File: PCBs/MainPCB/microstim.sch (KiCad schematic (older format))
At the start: 105 parts, among them J1 Conn_02x08_Counter_Clockwise, J2 Conn_Coaxial, J3 Conn_Coaxial, J4 Screw_Terminal_01x02, J5 Screw_Terminal_01x02, J6 Screw_Terminal_01x02, J7 Conn_Coaxial, J8 Screw_Terminal_01x02, J9 Conn_Coaxial, SW1 SW_Push, U1 Teensy3.5, U10 AD8276, U11 INA826, U12 DG509ACWE, U13 CC3-0512DF-E, U14 ISO7760, U15 ISO7341C, U16 L78L05_SO8, U17 AD5752, U18 AD7321, U19 AD1582, U2 CC3-0512DF-E, U20 OPA197, U21 AD8276, U22 INA826, U23 DG509ACWE, U3 ISO7760, U4 ISO7341C, U5 L78L05_SO8, U6 AD5752, U7 AD7321, U8 AD1582, U9 OPA197

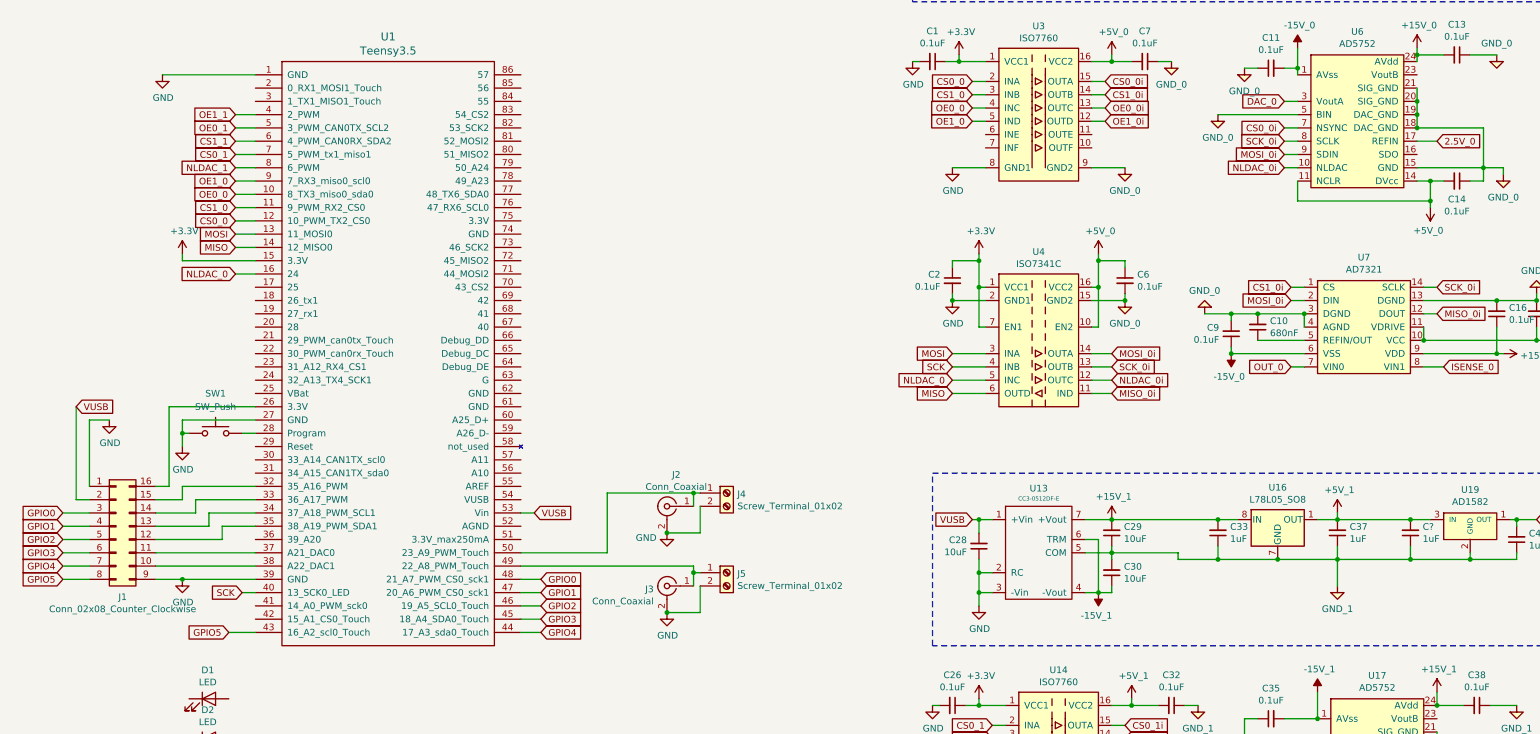
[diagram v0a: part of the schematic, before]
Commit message: getting darn close to done with layout.
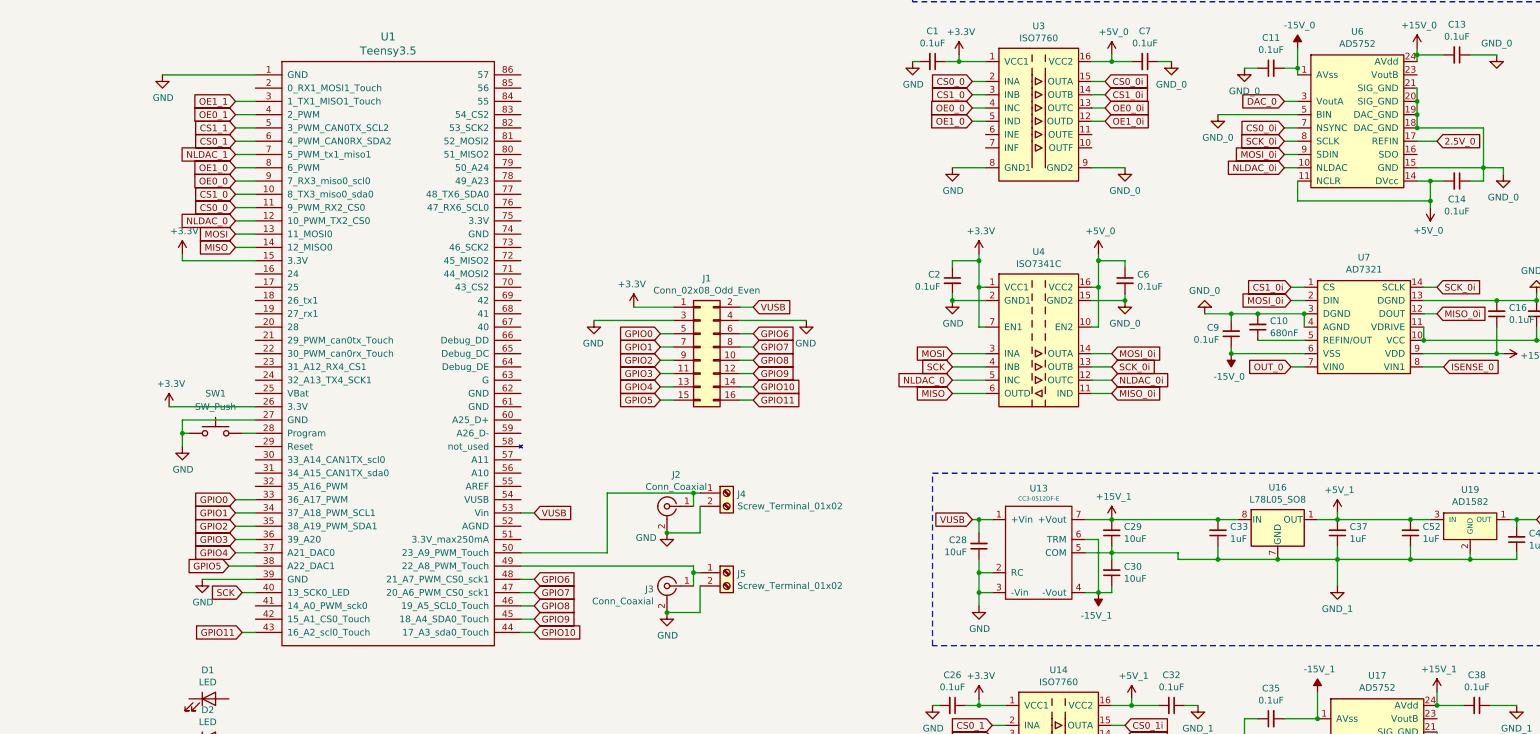
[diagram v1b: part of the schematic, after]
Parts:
- removed J1: Conn_02x08_Counter_Clockwise, Connector_Multicomp:Multicomp_MC9A22-1634_2x08_P2.54mm_Horizontal, symbol Connector_Generic:Conn_02x08_Counter_Clockwise
- added J1: Conn_02x08_Odd_Even, Connector_Multicomp:Multicomp_MC9A22-1634_2x08_P2.54mm_Horizontal, symbol Connector_Generic:Conn_02x08_Odd_Even
- gave numbers to parts that had none: 1
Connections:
- net +3V3: now also U1.26 (3.3V), J1.1 (Pin_1)
- net CS0_0: now also U1.11 (9_PWM_RX2_CS0); no longer U1.12 (10_PWM_TX2_CS0)
- net CS0_1: now also U1.6 (4_PWM_CAN0RX_SDA2); no longer U1.7 (5_PWM_tx1_miso1)
- net CS1_0: now also U1.10 (8_TX3_miso0_sda0); no longer U1.11 (9_PWM_RX2_CS0)
- net CS1_1: now also U1.5 (3_PWM_CAN0TX_SCL2); no longer U1.6 (4_PWM_CAN0RX_SDA2)
- net GND: now also J1.3 (Pin_3), J1.4 (Pin_4)
- net GPIO0: now also U1.33 (36_A17_PWM), J1.5 (Pin_5); no longer U1.48 (21_A7_PWM_CS0_sck1)
- net GPIO1: now also U1.34 (37_A18_PWM_SCL1), J1.7 (Pin_7); no longer U1.47 (20_A6_PWM_CS0_sck1)
- net GPIO2: now also U1.35 (38_A19_PWM_SDA1), J1.9 (Pin_9); no longer U1.46 (19_A5_SCL0_Touch)
- net GPIO3: now also U1.36 (39_A20), J1.11 (Pin_11); no longer U1.45 (18_A4_SDA0_Touch)
- net GPIO4: now also U1.37 (A21_DAC0), J1.13 (Pin_13); no longer U1.44 (17_A3_sda0_Touch)
- net GPIO5: now also U1.38 (A22_DAC1), J1.15 (Pin_15); no longer U1.43 (16_A2_scl0_Touch)
- net NLDAC_0: now also U1.12 (10_PWM_TX2_CS0); no longer U1.16 (24)
- net NLDAC_1: now also U1.7 (5_PWM_tx1_miso1); no longer U1.8 (6_PWM)
- net OE0_0: now also U1.9 (7_RX3_miso0_scl0); no longer U1.10 (8_TX3_miso0_sda0)
- net OE0_1: now also U1.4 (2_PWM); no longer U1.5 (3_PWM_CAN0TX_SCL2)
- net OE1_0: now also U1.8 (6_PWM); no longer U1.9 (7_RX3_miso0_scl0)
- net OE1_1: now also U1.3 (1_TX1_MISO1_Touch); no longer U1.4 (2_PWM)
- net VUSB: now also J1.2 (Pin_2)
- new net GPIO10: J1.14 (Pin_14), U1.44 (17_A3_sda0_Touch)
- new net GPIO11: J1.16 (Pin_16), U1.43 (16_A2_scl0_Touch)
- new net GPIO6: J1.6 (Pin_6), U1.48 (21_A7_PWM_CS0_sck1)
- new net GPIO7: J1.8 (Pin_8), U1.47 (20_A6_PWM_CS0_sck1)
- new net GPIO8: J1.10 (Pin_10), U1.46 (19_A5_SCL0_Touch)
- new net GPIO9: J1.12 (Pin_12), U1.45 (18_A4_SDA0_Touch)
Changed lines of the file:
@@
 Text GLabel 7350 1900 0    50   Input ~ 0
 OE0_0
-Text GLabel 1800 3150 0    50   Input ~ 0
+Text GLabel 1800 2750 0    50   Input ~ 0
 NLDAC_0
 $Comp
@@
 Wire Wire Line
 	8250 2350 8500 2350
-Text GLabel 1800 2650 0    50   Input ~ 0
+Text GLabel 1800 2550 0    50   Input ~ 0
 CS1_0
-Text GLabel 1800 2750 0    50   Input ~ 0
+Text GLabel 1800 2650 0    50   Input ~ 0
 CS0_0
 Wire Wire Line
@@
 Wire Wire Line
 	16750 4850 16900 4850
-Text GLabel 1800 2450 0    50   Input ~ 0
+Text GLabel 1800 2350 0    50   Input ~ 0
 OE1_0
-Text GLabel 1800 2550 0    50   Input ~ 0
+Text GLabel 1800 2450 0    50   Input ~ 0
 OE0_0
 Wire Wire Line
@@
 Wire Wire Line
 	1850 4350 1950 4350
-$Comp
-L Connector_Generic:Conn_02x08_Counter_Clockwise J1
-U 1 1 5CBED068
-P 900 5050
-F 0 "J1" H 950 4517 50  0000 C CNN
-F 1 "Conn_02x08_Counter_Clockwise" H 950 4426 50  0000 C CNN
-F 2 "Connector_Multicomp:Multicomp_MC9A22-1634_2x08_P2.54mm_Horizontal" H 900 5050 50  0001 C CNN
-F 3 "~" H 900 5050 50  0001 C CNN
-	1    900  5050
-	1    0    0    -1
-$EndComp
-Wire Wire Line
-	700  4250 700  4750
-Wire Wire Line
-	700  4850 600  4850
-Wire Wire Line
-	600  4850 600  4150
 Wire Wire Line
-	500  4950 700  4950
+	5000 3600 5100 3600
 Wire Wire Line
-	500  5050 700  5050
+	5000 3700 5100 3700
 Wire Wire Line
-	500  5150 700  5150
+	5000 3800 5100 3800
 Wire Wire Line
-	500  5250 700  5250
+	5000 3900 5100 3900
 Wire Wire Line
-	500  5350 700  5350
+	5000 4000 5100 4000
 Wire Wire Line
-	700  5450 500  5450
-Wire Wire Line
-	1950 5350 1200 5350
-Wire Wire Line
-	1200 5250 1950 5250
+	5100 4100 5000 4100
 Wire Wire Line
 	9950 150  10500 150
@@
 	1    0    0    -1
 $EndComp
-$Comp
-L power:GND #PWR01
-U 1 1 5C5D1E51
-P 850 4250
-F 0 "#PWR01" H 850 4000 50  0001 C CNN
-F 1 "GND" H 855 4077 50  0000 C CNN
-F 2 "" H 850 4250 50  0001 C CNN
-F 3 "" H 850 4250 50  0001 C CNN
-	1    850  4250
-	1    0    0    -1
-$EndComp
-Wire Wire Line
-	700  4250 850  4250
 Wire Wire Line
 	1950 4250 1400 4250
@@
 	1400 4350 1400 4450
 Wire Wire Line
-	1950 5050 1700 5050
-Wire Wire Line
-	1700 5050 1700 5150
-Wire Wire Line
-	1700 5150 1200 5150
-Wire Wire Line
-	1200 5050 1600 5050
-Wire Wire Line
-	1600 5050 1600 4950
-Wire Wire Line
-	1600 4950 1950 4950
-Wire Wire Line
-	1200 4950 1500 4950
-Wire Wire Line
-	1500 4950 1500 4850
-Wire Wire Line
-	1500 4850 1950 4850
-Wire Wire Line
-	1200 4850 1400 4850
-Wire Wire Line
-	1400 4850 1400 4750
-Wire Wire Line
-	1950 4750 1400 4750
-Wire Wire Line
-	1200 4750 1300 4750
-Wire Wire Line
-	1300 4750 1300 4150
-Wire Wire Line
 	1300 4150 1950 4150
-Text GLabel 600  4150 2    50   Input ~ 0
+Text GLabel 5700 3400 2    50   Input ~ 0
 VUSB
-Wire Wire Line
-	1200 5450 1400 5450
 $Comp
 L power:GND #PWR05
 U 1 1 5C9B26A7
-P 1400 5450
-F 0 "#PWR05" H 1400 5200 50  0001 C CNN
-F 1 "GND" H 1405 5277 50  0000 C CNN
-F 2 "" H 1400 5450 50  0001 C CNN
-F 3 "" H 1400 5450 50  0001 C CNN
-	1    1400 5450
-	1    0    0    -1
+P 4500 3500
+F 0 "#PWR05" H 4500 3250 50  0001 C CNN
+F 1 "GND" H 4505 3327 50  0000 C CNN
+F 2 "" H 4500 3500 50  0001 C CNN
+F 3 "" H 4500 3500 50  0001 C CNN
+	1    4500 3500
+	-1   0    0    -1
 $EndComp
-Connection ~ 1400 5450
-Wire Wire Line
-	1400 5450 1950 5450
-Text GLabel 500  5450 0    50   Input ~ 0
+Text GLabel 5000 4100 0    50   Input ~ 0
 GPIO5
-Text GLabel 500  5350 0    50   Input ~ 0
+Text GLabel 5000 4000 0    50   Input ~ 0
 GPIO4
-Text GLabel 500  5250 0    50   Input ~ 0
+Text GLabel 5000 3900 0    50   Input ~ 0
 GPIO3
-Text GLabel 500  5050 0    50   Input ~ 0
+Text GLabel 5000 3700 0    50   Input ~ 0
 GPIO1
-Text GLabel 500  5150 0    50   Input ~ 0
+Text GLabel 5000 3800 0    50   Input ~ 0
 GPIO2
-Text GLabel 500  4950 0    50   Input ~ 0
+Text GLabel 5000 3600 0    50   Input ~ 0
 GPIO0
-Text GLabel 1750 5850 0    50   Input ~ 0
+Text GLabel 1750 5350 0    50   Input ~ 0
 GPIO5
-Text GLabel 4100 5850 2    50   Input ~ 0
+Text GLabel 1800 5250 0    50   Input ~ 0
 GPIO4
-Text GLabel 4100 5750 2    50   Input ~ 0
+Text GLabel 1800 5150 0    50   Input ~ 0
 GPIO3
-Text GLabel 4100 5550 2    50   Input ~ 0
+Text GLabel 1800 4950 0    50   Input ~ 0
 GPIO1
-Text GLabel 4100 5650 2    50   Input ~ 0
+Text GLabel 1800 5050 0    50   Input ~ 0
 GPIO2
-Text GLabel 4100 5450 2    50   Input ~ 0
+Text GLabel 1800 4850 0    50   Input ~ 0
 GPIO0
 Wire Wire Line
-	1750 5850 1950 5850
+	1750 5350 1950 5350
 Wire Wire Line
-	3950 5850 4100 5850
+	1950 5250 1800 5250
 Wire Wire Line
-	4100 5750 3950 5750
+	1800 5150 1950 5150
 Wire Wire Line
-	3950 5650 4100 5650
+	1950 5050 1800 5050
 Wire Wire Line
-	4100 5550 3950 5550
+	1800 4950 1950 4950
 Wire Wire Line
-	3950 5450 4100 5450
-Text GLabel 1800 2350 0    50   Input ~ 0
-NLDAC_1
+	1950 4850 1800 4850
 Text GLabel 1800 2250 0    50   Input ~ 0
-CS0_1
+NLDAC_1
 Text GLabel 1800 2150 0    50   Input ~ 0
+CS0_1
+Text GLabel 1800 2050 0    50   Input ~ 0
 CS1_1
-Text GLabel 1800 1950 0    50   Input ~ 0
+Text GLabel 1800 1850 0    50   Input ~ 0
 OE1_1
-Text GLabel 1800 2050 0    50   Input ~ 0
+Text GLabel 1800 1950 0    50   Input ~ 0
 OE0_1
 Wire Wire Line
-	1800 2350 1950 2350
-Wire Wire Line
 	1800 2250 1950 2250
 Wire Wire Line
 	1800 2150 1950 2150
 Wire Wire Line
-	1800 1950 1950 1950
-Wire Wire Line
 	1800 2050 1950 2050
 Wire Wire Line
-	1800 3150 1950 3150
+	1800 1850 1950 1850
 Wire Wire Line
-	1800 2750 1950 2750
+	1800 1950 1950 1950
 Wire Wire Line
-	1950 2650 1800 2650
+	1800 2650 1950 2650
 Wire Wire Line
-	1800 2550 1950 2550
+	1950 2550 1800 2550
 Wire Wire Line
-	1950 2450 1800 2450
+	1800 2450 1950 2450
+Wire Wire Line
+	1950 2350 1800 2350
 Wire Wire Line
 	10750 3850 10900 3850
@@
 	10500 450  10950 450
 $Comp
-L Device:C_Small C?
+L Device:C_Small C52
 U 1 1 5C9B5470
 P 10650 5100
-F 0 "C?" H 10558 5054 50  0000 R CNN
+F 0 "C52" H 10558 5054 50  0000 R CNN
 F 1 "1uF" H 10558 5145 50  0000 R CNN
 F 2 "Capacitor_SMD:C_0603_1608Metric" H 10650 5100 50  0001 C CNN
@@
 Wire Wire Line
 	10650 5300 11100 5300
+Wire Wire Line
+	1800 2750 1950 2750
+Text GLabel 5700 4000 2    50   Input ~ 0
+GPIO10
+Text GLabel 5700 3900 2    50   Input ~ 0
+GPIO9
+Text GLabel 5700 3700 2    50   Input ~ 0
+GPIO7
+Text GLabel 5700 3800 2    50   Input ~ 0
+GPIO8
+Text GLabel 5700 3600 2    50   Input ~ 0
+GPIO6
+$Comp
+L power:GND #PWR0110
+U 1 1 5CC7B82D
+P 1550 5450
+F 0 "#PWR0110" H 1550 5200 50  0001 C CNN
+F 1 "GND" H 1555 5277 50  0000 C CNN
+F 2 "" H 1550 5450 50  0001 C CNN
+F 3 "" H 1550 5450 50  0001 C CNN
+	1    1550 5450
+	1    0    0    -1
+$EndComp
+Wire Wire Line
+	1550 5450 1950 5450
+Wire Wire Line
+	5700 3400 5600 3400
+$Comp
+L power:+3.3V #PWR0111
+U 1 1 5D1270A2
+P 1300 4150
+F 0 "#PWR0111" H 1300 4000 50  0001 C CNN
+F 1 "+3.3V" H 1315 4323 50  0000 C CNN
+F 2 "" H 1300 4150 50  0001 C CNN
+F 3 "" H 1300 4150 50  0001 C CNN
+	1    1300 4150
+	1    0    0    -1
+$EndComp
+Text GLabel 5700 4100 2    50   Input ~ 0
+GPIO11
+Wire Wire Line
+	5600 4100 5700 4100
+Wire Wire Line
+	5600 4000 5700 4000
+Wire Wire Line
+	5600 3900 5700 3900
+Wire Wire Line
+	5600 3800 5700 3800
+Wire Wire Line
+	5600 3700 5700 3700
+Wire Wire Line
+	5600 3600 5700 3600
+$Comp
+L power:+3.3V #PWR0112
+U 1 1 5D3D870A
+P 4800 3400
+F 0 "#PWR0112" H 4800 3250 50  0001 C CNN
+F 1 "+3.3V" H 4815 3573 50  0000 C CNN
+F 2 "" H 4800 3400 50  0001 C CNN
+F 3 "" H 4800 3400 50  0001 C CNN
+	1    4800 3400
+	-1   0    0    -1
+$EndComp
+Text GLabel 4050 5850 2    50   Input ~ 0
+GPIO10
+Text GLabel 4050 5750 2    50   Input ~ 0
+GPIO9
+Text GLabel 4050 5550 2    50   Input ~ 0
+GPIO7
+Text GLabel 4050 5650 2    50   Input ~ 0
+GPIO8
+Text GLabel 4050 5450 2    50   Input ~ 0
+GPIO6
+Text GLabel 1850 5850 0    50   Input ~ 0
+GPIO11
+Wire Wire Line
+	4050 5450 3950 5450
+Wire Wire Line
+	4050 5550 3950 5550
+Wire Wire Line
+	4050 5650 3950 5650
+Wire Wire Line
+	4050 5750 3950 5750
+Wire Wire Line
+	4050 5850 3950 5850
+Wire Wire Line
+	1850 5850 1950 5850
+Wire Wire Line
+	4800 3400 5100 3400
+$Comp
+L Connector_Generic:Conn_02x08_Odd_Even J1
+U 1 1 5DFCF206
+P 5300 3700
+F 0 "J1" H 5350 4217 50  0000 C CNN
+F 1 "Conn_02x08_Odd_Even" H 5350 4126 50  0000 C CNN
+F 2 "Connector_Multicomp:Multicomp_MC9A22-1634_2x08_P2.54mm_Horizontal" H 5300 3700 50  0001 C CNN
+F 3 "~" H 5300 3700 50  0001 C CNN
+	1    5300 3700
+	1    0    0    -1
+$EndComp
+Wire Wire Line
+	4500 3500 5100 3500
+$Comp
+L power:GND #PWR0113
+U 1 1 5E353902
+P 6100 3500
+F 0 "#PWR0113" H 6100 3250 50  0001 C CNN
+F 1 "GND" H 6105 3327 50  0000 C CNN
+F 2 "" H 6100 3500 50  0001 C CNN
+F 3 "" H 6100 3500 50  0001 C CNN
+	1    6100 3500
+	-1   0    0    -1
+$EndComp
+Wire Wire Line
+	5600 3500 6100 3500
 $EndSCHEMATC

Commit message: finished layout, schematic+pcb pdfs, BOM. need to do panels.
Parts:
- removed J4, J5: Screw_Terminal_01x02, microstim:1-2834016-2 _TERM_BLK_2P_SIDE_ENT_2.54MM_PCB, symbol Connector:Screw_Terminal_01x02
- added R15, R16: 200, Resistor_SMD:R_0603_1608Metric, symbol Device:R_US
- D1, D2: footprint LED_THT:LED_D5.0mm_Horizontal_O1.27mm_Z3.0mm -> microstim:LED_D5.0mm_Horizontal_O1.27mm_Z3.0mm_pinSwapped
- SW1: footprint Button_Switch_SMD:SW_SPST_EVPBF -> microstim:EVQ-PF303K
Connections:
- net +3V3: now also J1.3 (Pin_3); no longer J1.1 (Pin_1)
- net GND: now also D1.1 (K), D2.1 (K), J1.1 (Pin_1); no longer J1.3 (Pin_3)
- net GPIO10: now also U1.42 (15_A1_CS0_Touch); no longer U1.44 (17_A3_sda0_Touch)
- net GPIO11: now also U1.41 (14_A0_PWM_sck0); no longer U1.43 (16_A2_scl0_Touch)
- net GPIO6: now also U1.46 (19_A5_SCL0_Touch); no longer U1.48 (21_A7_PWM_CS0_sck1)
- net GPIO7: now also U1.45 (18_A4_SDA0_Touch); no longer U1.47 (20_A6_PWM_CS0_sck1)
- net GPIO8: now also U1.44 (17_A3_sda0_Touch); no longer U1.46 (19_A5_SCL0_Touch)
- net GPIO9: now also U1.43 (16_A2_scl0_Touch); no longer U1.45 (18_A4_SDA0_Touch)
- net at U12.11 (S3B): no longer U12.6 (S3A)
- net at R7.1, U12.4 (S1A), U12.7 (S4A): now also U12.6 (S3A)
- net at U23.11 (S3B): no longer U23.6 (S3A)
- net at R14.2, U23.4 (S1A), U23.7 (S4A): now also U23.6 (S3A)
- net at D1.2 (A): now also R15.1
- net at D2.2 (A): now also R16.1
- new net: R16.2, U1.47 (20_A6_PWM_CS0_sck1)
- new net: R15.2, U1.48 (21_A7_PWM_CS0_sck1)
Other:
- note added: "Max current output (0ohm load) is (+/-10V)/3k = +- 3.33mA.\nCurrent resolution is 20V/2^16/3k = 0.1uA\nMax voltage output (infinite load) is 40/43*14.8V = +/-13.76V"
- note added: "OE0 OE1 Output \n\n 0 0 VOLTAGE \n 1 0 CURRENT \n 0 1 High-Z \n 1 1 GND"
- note added: "Stim channel 0"
- note added: "Stim channel 1"
- note added: "gain is Rsense*(1+49.4k/Rg) = 100*(1+49.4k/1.8k) = 2.87 mV/uA\nVoltage output range is thus +-3333*0.00287 = +-9.57V\noutput needs to be within +-10V\ncurrent sensing resolution is 10000 mV / 2^12 / (2.87mV/uA) = 0.85uA\n\n"
- note removed: "Max current output (0ohm load) is 10V/3k = +- 3.33mA.\nCurrent resolution is 20V/2^16/3k = 0.1uA\nMax voltage output (infinite load) is 40/43*15V = +/-13.95V"
- note removed: "OE0 OE1 Output Input (ADC)\n\n 0 0 VOLTAGE OUT0\n 1 0 CURRENT OUT0\n 0 1 CURRENT ISENSE0\n 1 1 GND ISENSE0"
- note removed: "gain is Rsense*(1+49.4k/Rg) = 100*(1+49.4k/1.8k) = 2.84 mV/uA\nVoltage output range is thus +-3333*0.00284 = +-9.48V\noutput needs to be within +-10V\ncurrent sensing resolution is 10000 mV / 2^12 / (2.84mV/uA) = 0.86uA\n\n"
- moved on the sheet: C1, C10, C11, C12, C13, C14, C15, C16, C17, C18, C19, C2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
